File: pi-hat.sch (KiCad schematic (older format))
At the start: 20 parts, among them J1 Raspberry_Pi_2_3, J2 Conn_SPI, J4 Conn_01x08, J5 USB_B, J6 Conn_01x02, J7 USB_OUT, J9 Conn_01x02, Q1 Q_NMOS_GDS, Q5 Q_NMOS_GDS, U2 MAX98357

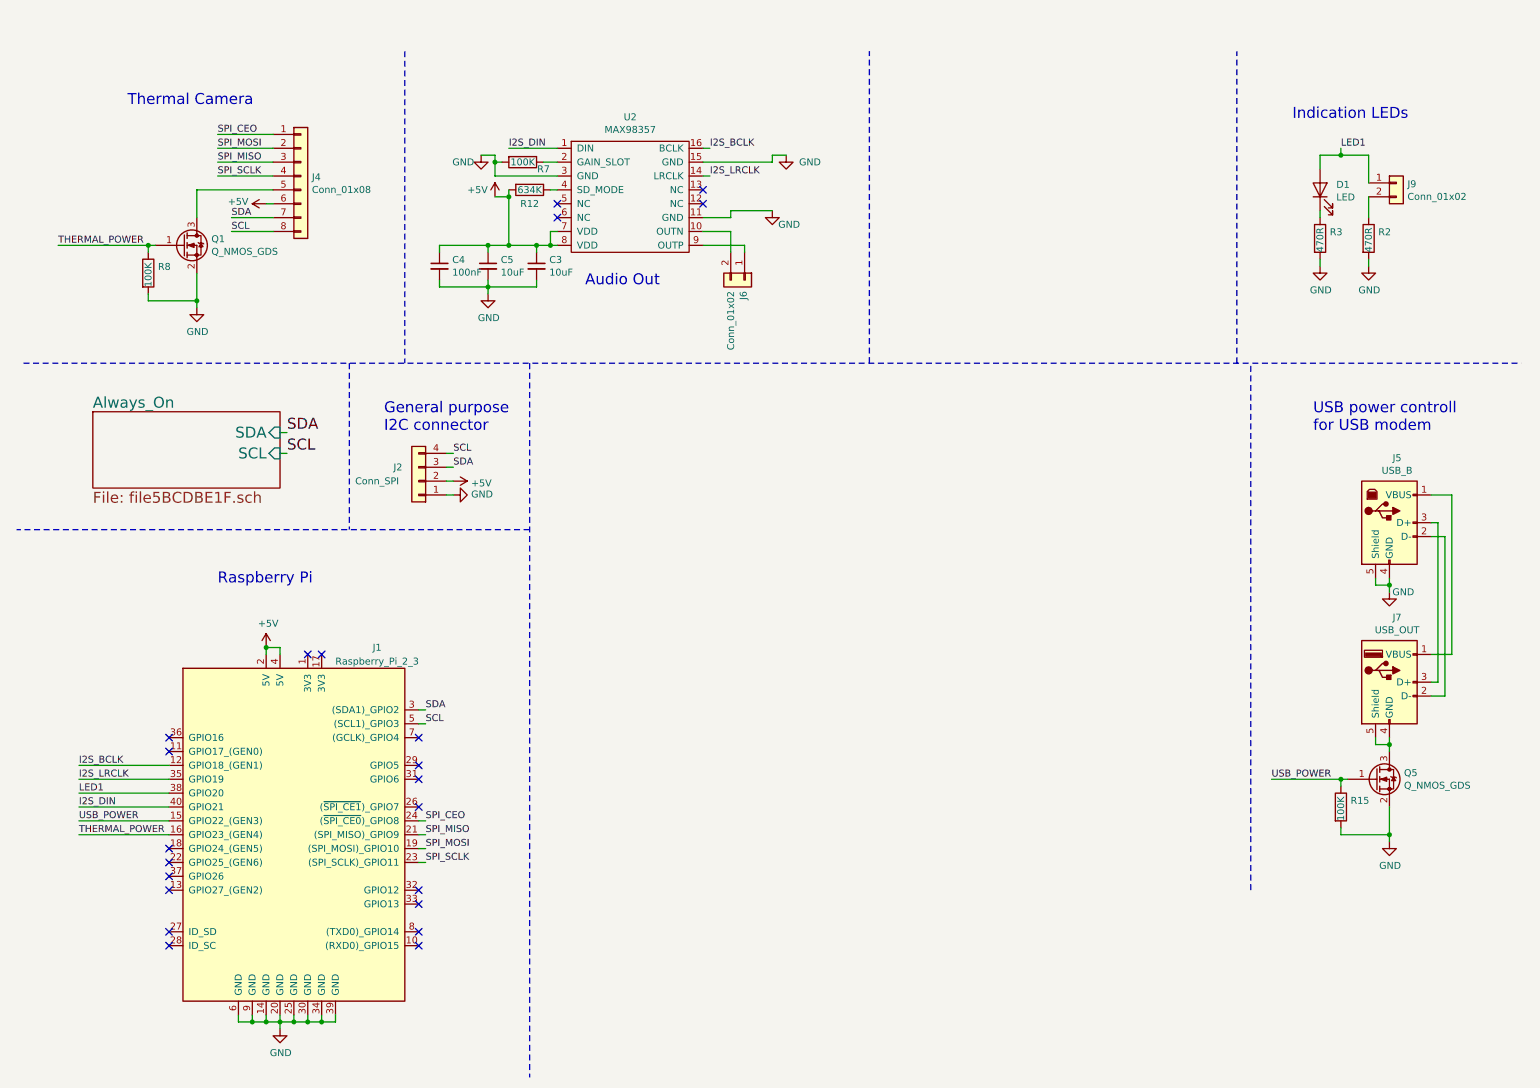
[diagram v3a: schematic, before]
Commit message: Updated to version 0.3
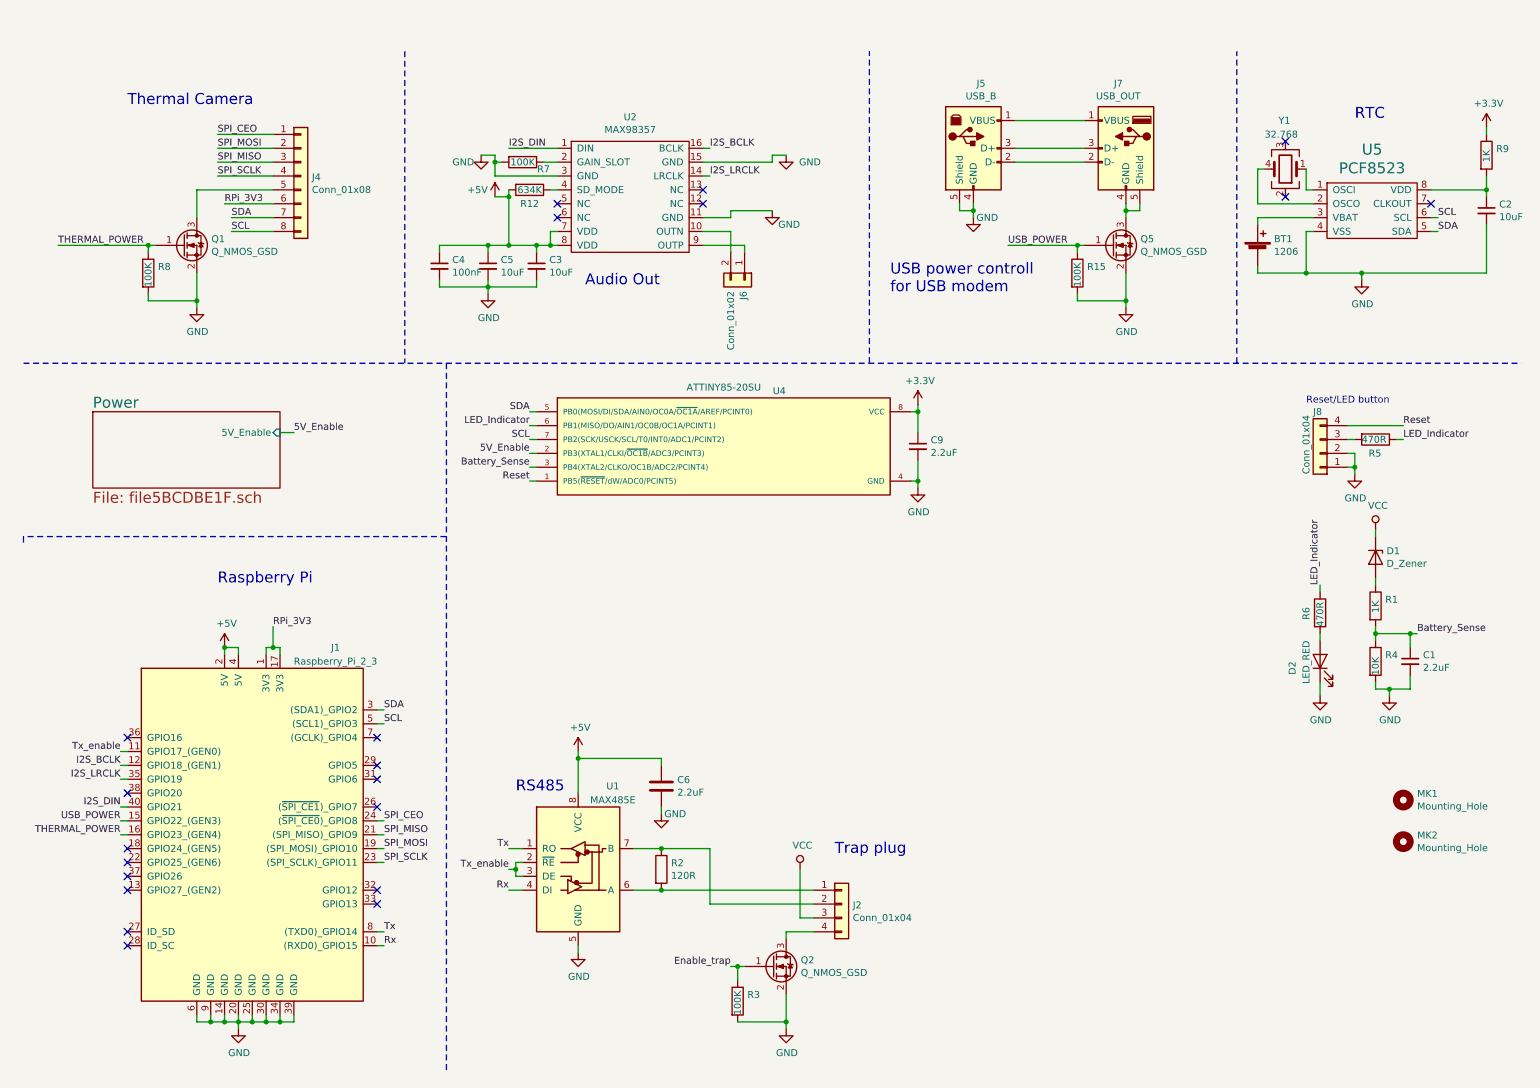
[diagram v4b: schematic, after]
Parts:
- removed D1: LED, LEDs:LED_0603_HandSoldering, symbol pi-hat-rescue:LED-Device-pi-hat-rescue
- removed J2: Conn_SPI, Connectors_JST:JST_XH_B04B-XH-A_04x2.50mm_Straight, symbol pi-hat-rescue:Conn_01x04-Connector_Generic-pi-hat-rescue
- removed J9: Conn_01x02, Connectors_JST:JST_XH_B02B-XH-A_02x2.50mm_Straight, symbol conn:Conn_01x02
- removed R2, R3: 470R, Resistors_SMD:R_0603_HandSoldering, symbol pi-hat-rescue:R-Device-pi-hat-rescue
- added BT1: 1206, pi-hat-footprints:CR1220, symbol device:Battery_Cell
- added C1, C9: 2.2uF, Capacitors_SMD:C_0603, symbol device:C_Small
- added C2: 10uF, Capacitors_SMD:C_0805, symbol device:C_Small
- added C6: 2.2uF, Capacitors_SMD:C_0603, symbol Device:C
- added D1: D_Zener, Diodes_SMD:D_SOD-323, symbol device:D_Zener
- added D2: LED_RED, LEDs:LED_0603, symbol pi-hat-rescue:LED-Device-pi-hat-rescue
- added J2, J8: Conn_01x04, Connectors_JST:JST_XH_B04B-XH-A_04x2.50mm_Straight, symbol conn:Conn_01x04
- added MK1, MK2: Mounting_Hole, Mounting_Holes:MountingHole_3mm_Pad, symbol Mechanical:Mounting_Hole
- added Q2: Q_NMOS_GSD, TO_SOT_Packages_SMD:SOT-23, symbol pi-hat-rescue:Q_NMOS_GSD-Device-pi-hat-rescue
- added R1, R9: 1K, Resistors_SMD:R_0603, symbol device:R
- added R2: 120R, Resistors_SMD:R_0603, symbol Device:R
- added R3: 100K, Resistors_SMD:R_0603, symbol Device:R
- added R4: 10K, Resistors_SMD:R_0603, symbol device:R
- added R5, R6: 470R, Resistors_SMD:R_0603, symbol pi-hat-rescue:R-Device-pi-hat-rescue
- added U1: MAX485E, Housings_SSOP:MSOP-8_3x3mm_Pitch0.65mm, symbol interface:MAX485E
- added U4: ATTINY85-20SU, Housings_DIP:DIP-8_W7.62mm_Socket, symbol pi-hat-rescue:ATTINY85-20SU-pi-hat-cache-pi-hat-rescue
- added U5: PCF8523, Housings_SOIC:SOIC-8_3.9x4.9mm_Pitch1.27mm, symbol cacophony-pi-hat:PCF8523
- added Y1: 32.768, Crystals:Crystal_SMD_SeikoEpson_MC306-4pin_8.0x3.2mm, symbol device:Crystal_GND23
- C3, C4, C5: footprint Capacitors_SMD:C_0805_HandSoldering -> Capacitors_SMD:C_0805
- J4: OPL (none) -> B8B-XH-A(LF)(SN)
- J6: OPL (none) -> 1725656
- Q1, Q5: value Q_NMOS_GDS -> Q_NMOS_GSD; footprint TO_SOT_Packages_SMD:SC-59_Handsoldering -> TO_SOT_Packages_SMD:SOT-23; Digikey 785-1015-1-ND -> 785-1009-1-ND; Link https://www.digikey.com/product-detail/en/alpha-omega-semiconductor-inc/AO3422/785-1015-1-ND/1855957 -> https://www.digikey.com/product-detail/en/alpha-omega-semiconductor-inc/AO3414/785-1009-1-ND/1855951; MPN AO3422 -> AO3414
- R12: footprint Resistors_SMD:R_0603_HandSoldering -> Resistors_SMD:R_0603
- R15, R7, R8: footprint Resistors_SMD:R_0603_HandSoldering -> Resistors_SMD:R_0603; OPL RC0603JR-07100KL -> (none)
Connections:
- net +5V: now also C6.1, U1.8 (VCC); no longer J4.6 (Pin_6)
- net GND: now also BT1.2 (-), C1.2, C2.2, C6.2, C9.2, D2.1 (K), J8.1 (Pin_1), J8.2 (Pin_2), Q2.2 (S), R3.2, R4.2, U1.5 (GND), U4.4 (GND), U5.4 (VSS)
- net SCL: now also U4.7 (PB2(SCK/USCK/SCL/T0/INT0/ADC1/PCINT2)), U5.6 (SCL)
- net SDA: now also U4.5 (PB0(MOSI/DI/SDA/AIN0/OC0A/~OC1A~/AREF/PCINT0)), U5.5 (SDA)
- net RPi_3V3: now reaches J1.1 (3V3)
- net RPi_3V3: now also J1.17 (3V3), J4.6 (Pin_6)
- net Rx: now reaches J1.10 ((RXD0)_GPIO15)
- net Rx: now also U1.4 (DI)
- net Tx_enable: now reaches J1.11 (GPIO17_(GEN0))
- net Tx_enable: now also U1.2 (~RE), U1.3 (DE)
- net Tx: now reaches J1.8 ((TXD0)_GPIO14)
- net Tx: now also U1.1 (RO)
- net LED1: no longer names the net of J1.38 (GPIO20)
- new net: J2.1 (Pin_1), R2.2, U1.6 (A)
- new net: J2.2 (Pin_2), R2.1, U1.7 (B)
- new net: J2.4 (Pin_4), Q2.3 (D)
- new net: D2.2 (A), R6.2
- new net: D1.2 (A), R1.1
- new net: J8.3 (Pin_3), R5.2
- new net: U5.1 (OSCI), Y1.1
- new net: U5.2 (OSCO), Y1.4
- new net: BT1.1 (+), U5.3 (VBAT)
- new net: C2.1, R9.2, U5.8 (VDD)
- new net +3V3: C9.1, R9.1, U4.8 (VCC)
- new net 5V_Enable: U4.2 (PB3(XTAL1/CLKI/~OC1B~/ADC3/PCINT3))
- new net Battery_Sense: C1.1, R1.2, R4.1, U4.3 (PB4(XTAL2/CLKO/OC1B/ADC2/PCINT4))
- new net Enable_trap: Q2.1 (G), R3.1
- new net LED_Indicator: R5.1, R6.1, U4.6 (PB1(MISO/DO/AIN1/OC0B/OC1A/PCINT1))
- new net Reset: J8.4 (Pin_4), U4.1 (PB5(~RESET~/dW/ADC0/PCINT5))
- new net VCC: D1.1 (K), J2.3 (Pin_3)
- no-connect marks 22 -> 21
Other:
- note added: "RS485"
- note added: "RTC"
- note added: "Reset/LED button"
- note added: "Trap plug"
- note removed: "General purpose \nI2C connector"
- note removed: "Indication LEDs"
- moved on the sheet: J1, J5, J7, Q5, R15
